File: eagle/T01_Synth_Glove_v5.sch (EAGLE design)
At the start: 79 parts, among them IC1 317T, SW1 RESET_BUTTON, U1 ATMEGA328P, U2 ZLDO1117, U4 LT1013

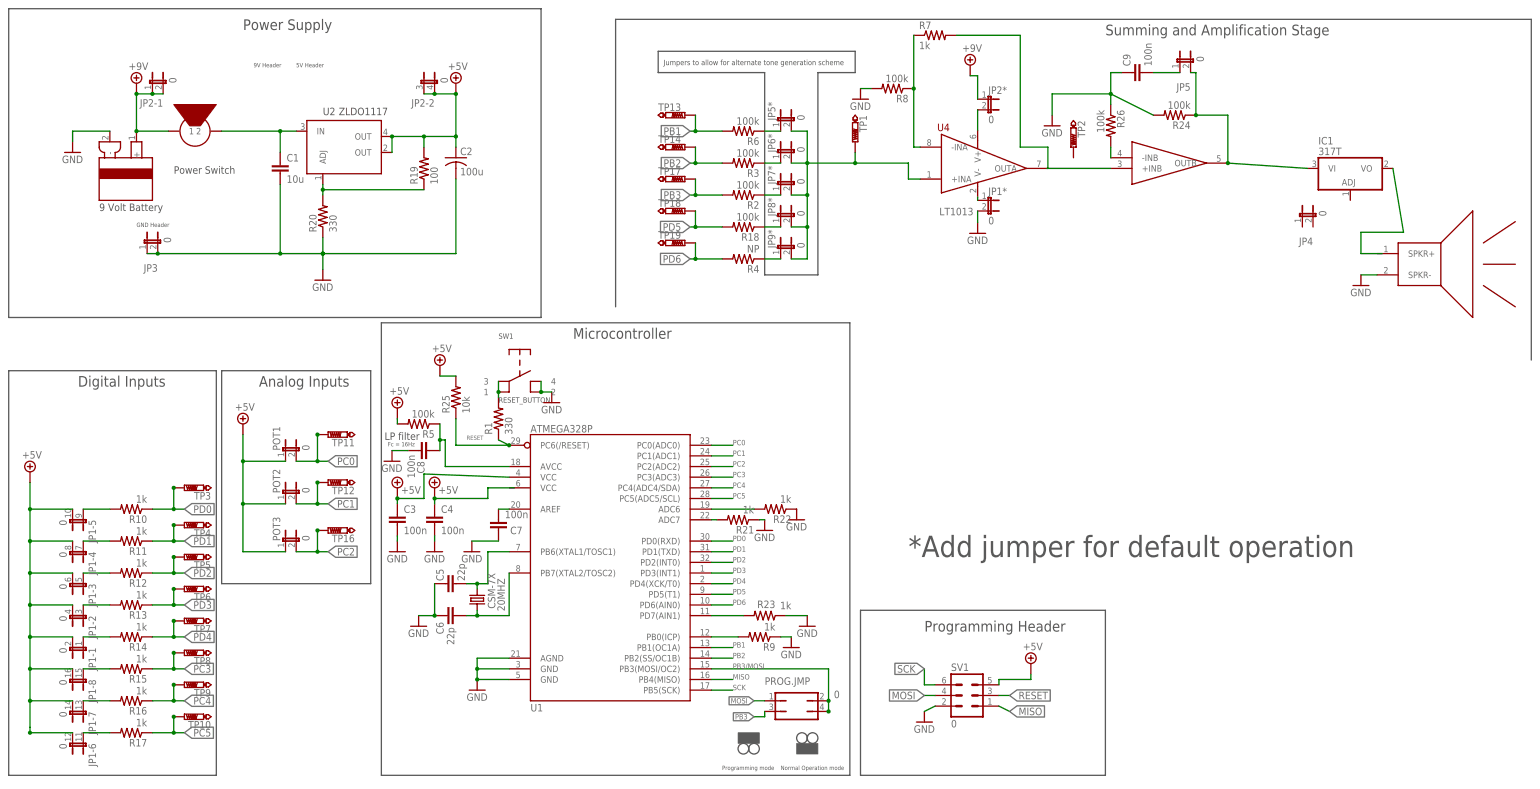
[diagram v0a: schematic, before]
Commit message: issue 5 and greenberg requsts
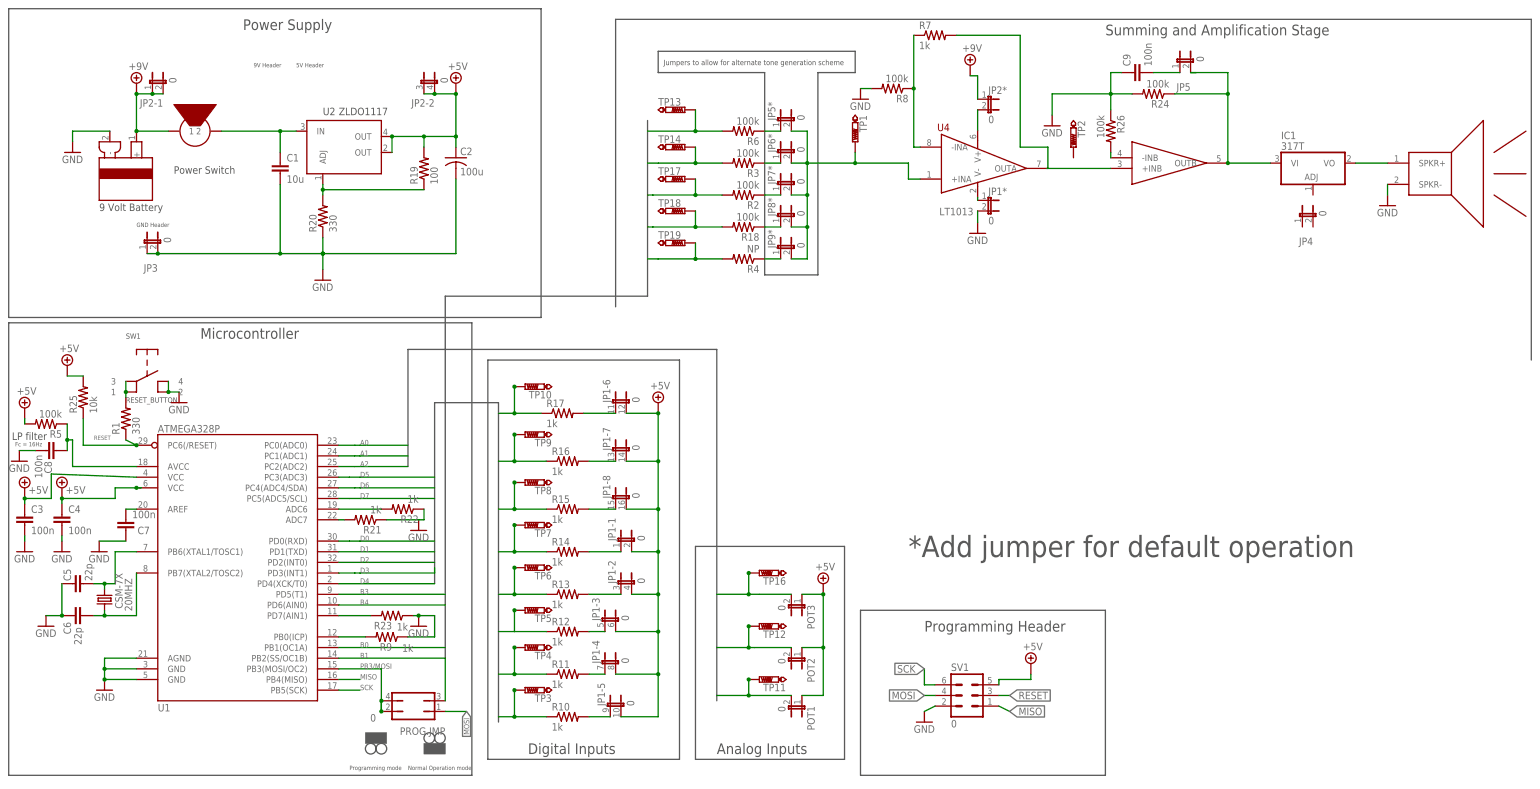
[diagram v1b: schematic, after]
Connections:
- net PB1 renamed B0
- net PC0 renamed A0
- net PC1 renamed A1
- net PC2 renamed A2
- net PC3 renamed D5
- net PC4 renamed D6
- net PC5 renamed D7
- net PD0 renamed D0
- net PD1 renamed D1
- net PD2 renamed D2
- net PD3 renamed D3
- net PD4 renamed D4
- net PD5 renamed B3
- net PD6 renamed B4
- removed net PB2: R3.2, TP14.TP, U1.PB2(SS/OC1B)
- removed net PB3: PROG.JMP.3, R2.2, TP17.TP
- new net B1: R2.2, R3.2, TP14.TP, TP17.TP, U1.PB2(SS/OC1B)
- new net B2: PROG.JMP.3
- net +5V: now also U1.VCC@2
- net N$31: now also U$1.SPKR+
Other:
- moved on the sheet: 20MHZ, C3, C4, C5, C6, C7, C8, IC1, JP1-1, JP1-2, JP1-3, JP1-4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
